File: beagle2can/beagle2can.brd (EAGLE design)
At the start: 160 x 100 mm, 36 parts, among them IC1 R-785.0-0.5, P1 39-30-04?_S, U1 TXB0108PWR

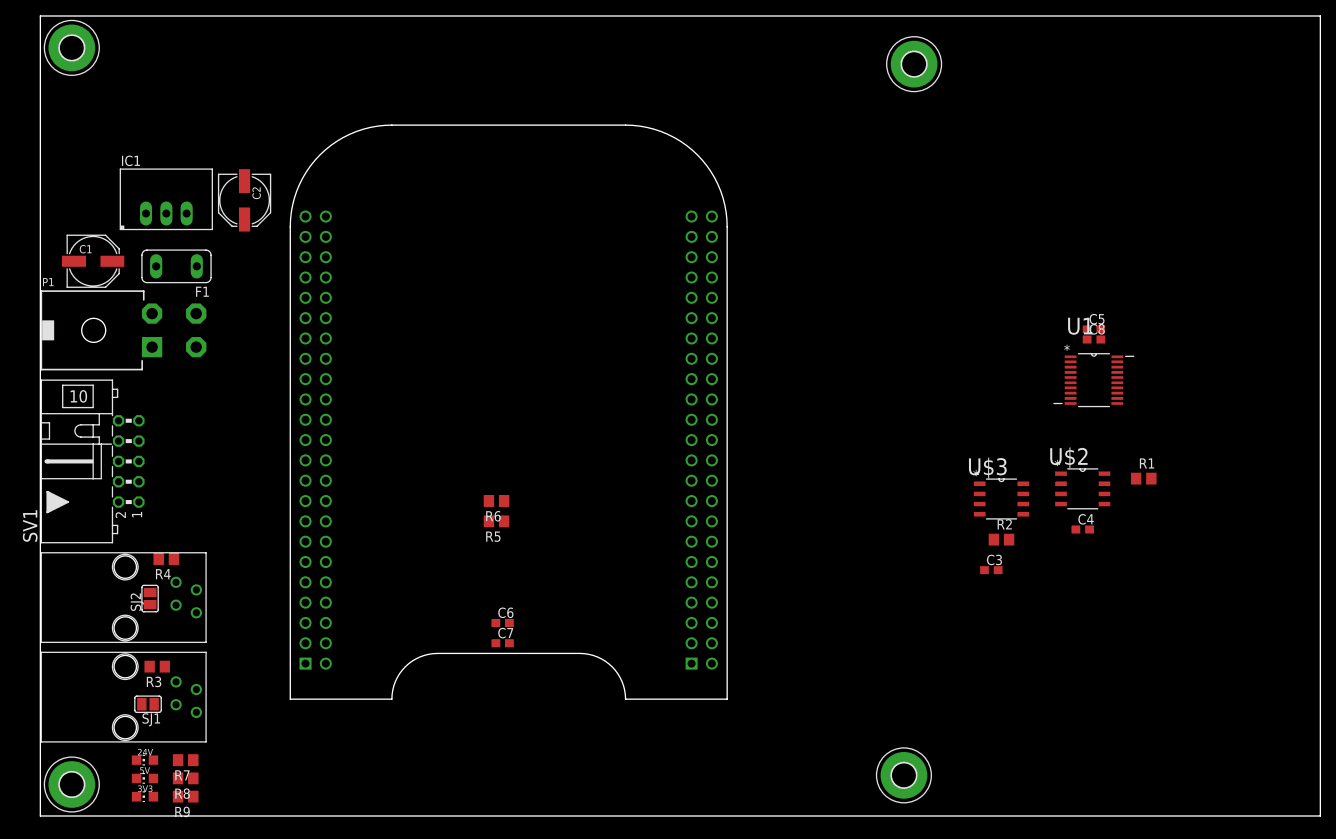
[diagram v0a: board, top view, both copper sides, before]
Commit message: beagle2can layout finished
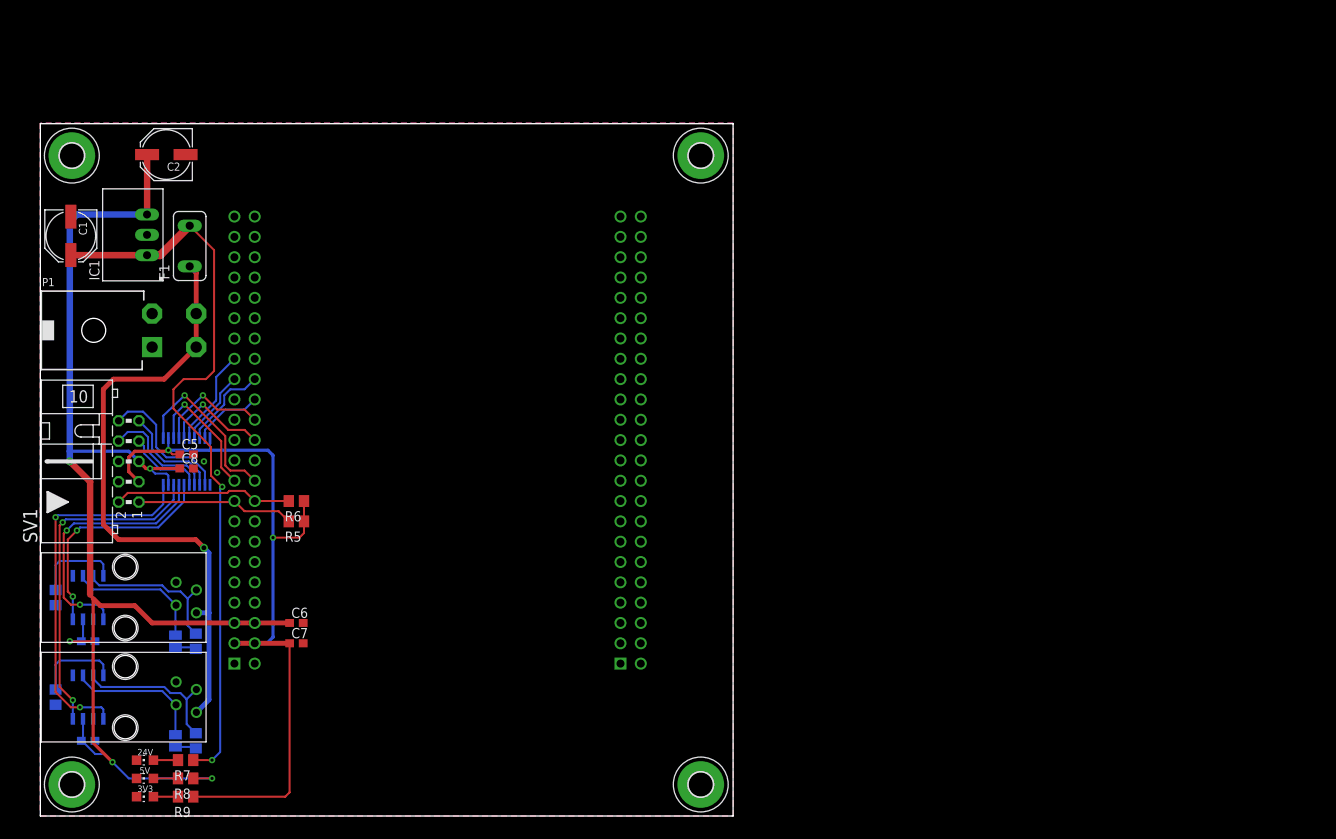
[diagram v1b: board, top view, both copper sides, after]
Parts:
- U$1: device adafruit:BEAGLEBONE_SHIELD -> ownParts:BEAGLEBONE_SHIELD
- moved R1 138.7 mm to (1.91, 14.9), flipped to the bottom, turned to 90 degrees
- moved C4 127.1 mm to (5.97, 9.40), flipped to the bottom, turned to 180 degrees
- moved U$2 127.0 mm to (5.97, 14.9), flipped to the bottom, turned to 90 degrees
- moved R2 118.5 mm to (1.91, 27.3), flipped to the bottom, turned to 90 degrees
- moved U$3 114.8 mm to (5.97, 27.3), flipped to the bottom, turned to 90 degrees
- moved C8 114.6 mm to (18.3, 43.4)
- moved C5 114.5 mm to (18.3, 45.2)
- moved U1 113.9 mm to (18.3, 44.3), flipped to the bottom, turned to 270 degrees
- moved C3 113.3 mm to (5.97, 21.8), flipped to the bottom, turned to 180 degrees
- moved H3 29.0 mm to (82.5, 82.5)
- moved C6 25.8 mm to (32.0, 24.1)
- moved C7 25.8 mm to (32.0, 21.6)
- moved H4 25.4 mm to (82.5, 3.94)
- moved R5 25.0 mm to (32.0, 36.8)
- moved R6 25.0 mm to (32.0, 39.4)
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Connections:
- net CON_24V: now also RJ_1.P$4, RJ_2.P$4
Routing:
- net +5V: track 0.00 -> 165.2 mm, vias 0 -> 5
- net +3V3: track 0.00 -> 98.2 mm, vias 0 -> 2
- net +24V: track 0.00 -> 94.1 mm, vias 0 -> 2
- net CON_24V: track 0.00 -> 78.0 mm, vias 0 -> 1
- net CAN0_TX_5V: track 0.00 -> 46.5 mm, vias 0 -> 2
- net CAN0_RX_5V: track 0.00 -> 42.3 mm, vias 0 -> 2
- net CAN1_TX_5V: track 0.00 -> 32.9 mm, vias 0 -> 2
- net CAN1_RX_5V: track 0.00 -> 28.8 mm, vias 0 -> 2
- net I2C1_SDA: track 0.00 -> 22.4 mm
- net CAN0_TX: track 0.00 -> 21.8 mm, vias 0 -> 1
- net I2C1_SCL: track 0.00 -> 19.8 mm
- net CAN0_H: track 0.00 -> 19.6 mm
- net CAN1_H: track 0.00 -> 19.6 mm
- net SPI1_CS_5V: track 0.00 -> 17.7 mm
- net CAN0_L: track 0.00 -> 17.3 mm
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- added copper zone on layer 1, net GND
- added copper zone on layer 16, net GND
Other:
- board size 160 x 100 mm -> 86.6 x 86.5 mm
